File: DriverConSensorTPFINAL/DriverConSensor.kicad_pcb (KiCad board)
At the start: 2 copper layers, 77 x 67 mm, 51 parts, among them J1 PULS1, J2 PULS2, J3 MotorT2, J4 MotorT1, J5 VIn+12, J6 Contac12V, J7 GND, K1 Switch de Encendido, K2 FRS10CS10-12V, K3 FRS10CS10-12V, Q1 BC337, Q2 BC337, SW1 SW_DIP_x06, U1 PIC12F675-IP, U2 L78L05, U3 ACS714T-30A

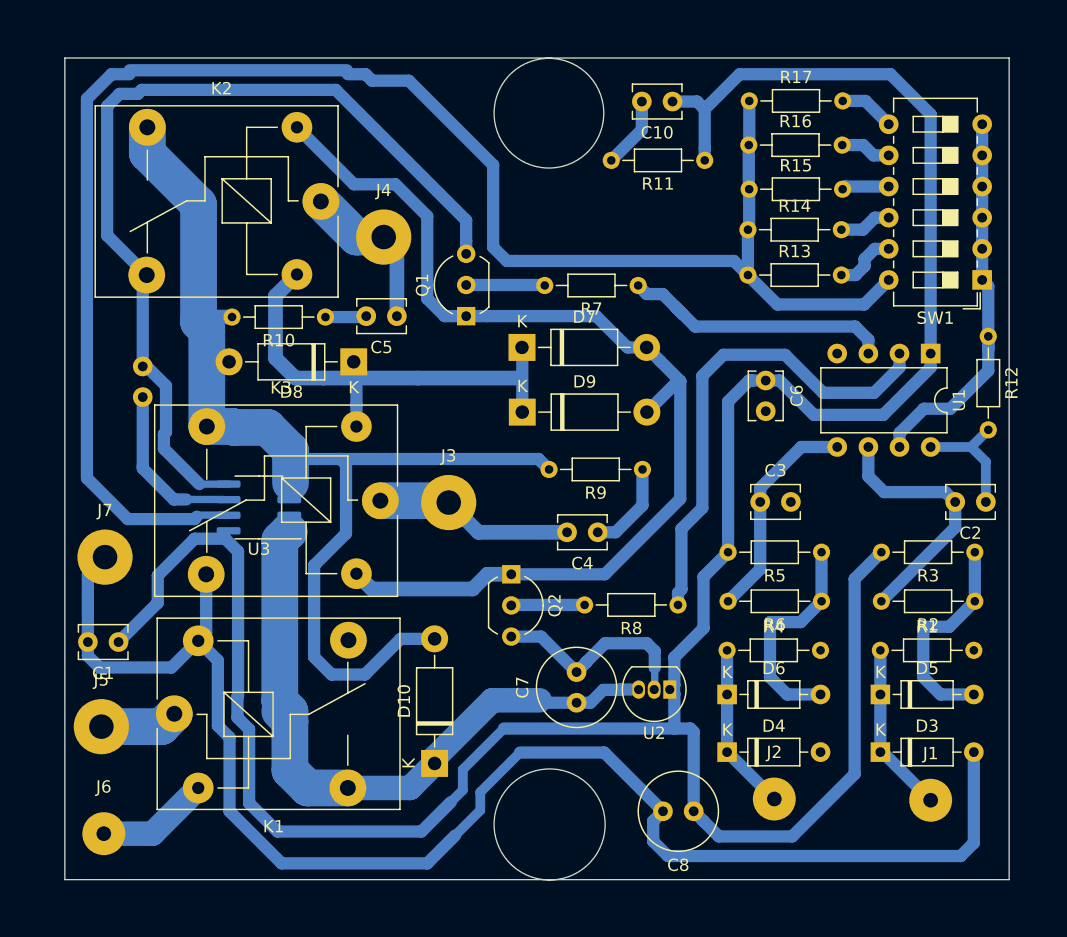
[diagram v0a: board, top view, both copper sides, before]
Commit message: actual2
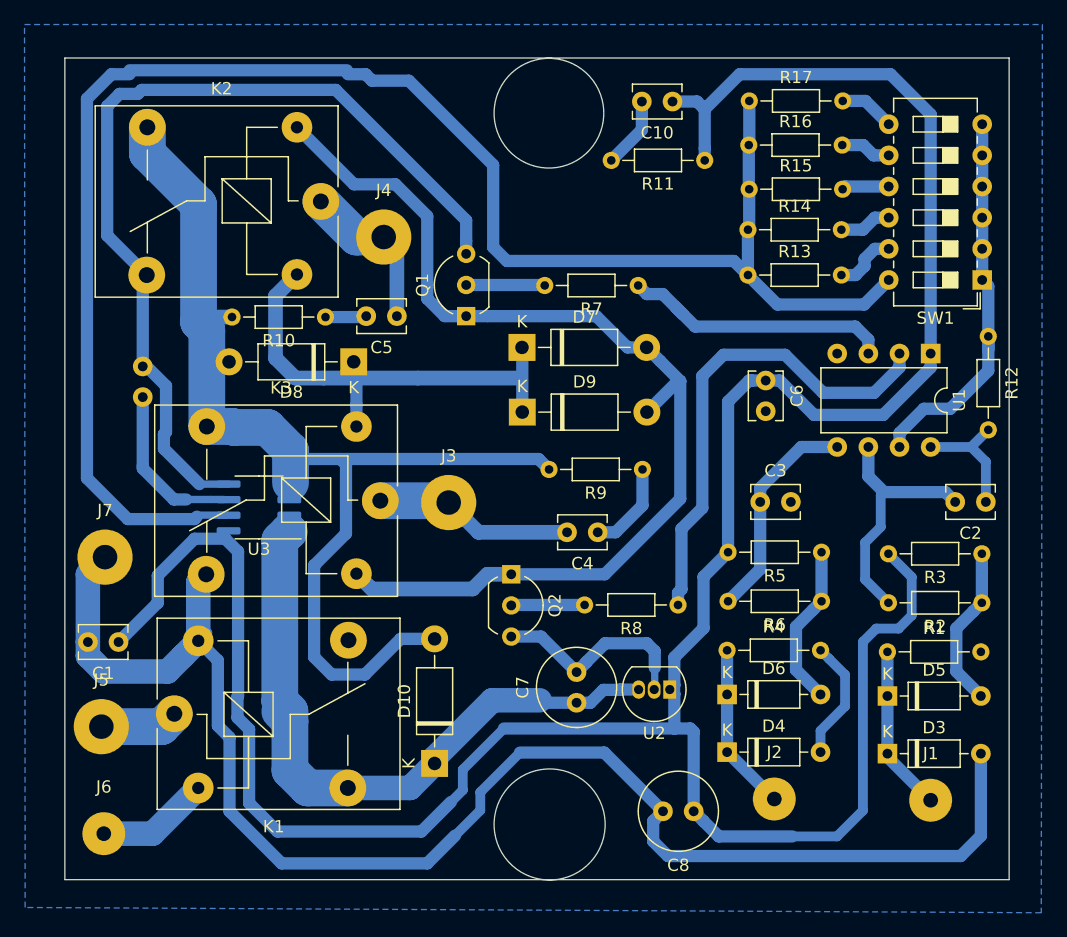
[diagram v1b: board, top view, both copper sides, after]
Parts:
- moved R2 0.59 mm to (187.8, 107.4)
- moved R3 0.59 mm to (187.8, 103.4)
- moved D3 0.59 mm to (180.1, 119.7)
- moved D5 0.59 mm to (180.1, 115.0)
- moved R1 0.59 mm to (180.1, 111.4)
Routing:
- net GND: track 228.2 -> 239.4 mm
- net +5V: track 216.4 -> 221.3 mm
- net Net-(D6-Pad2): track 18.1 -> 13.3 mm
- net Net-(D5-Pad2): track 17.8 -> 13.3 mm
- added copper zone on B.Cu, net GND
